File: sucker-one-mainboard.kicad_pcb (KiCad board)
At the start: 4 copper layers, 79.4 x 63 mm, 114 parts, among them J1 JST NC Valve, J10 JST Motor, J11 User Interface Module, J12 SWD, J2 JST NO Valve, J3 6P4C, J4 JST 3 Way Valve, J5 AUX SPI, J6 AUX I2C, Q1 BSS138, Q2 BSS138, Q3 BSS138, Q4 DMN15H310SE-13, SW1 Power Switch, SW2 Reset, U1 LD1117S33TR, U2 TPS61087DRCR, U3 STM32F103RBTx, U4 2SMPP-03, U5 INA125UA, Y1 8MHz(16pf)

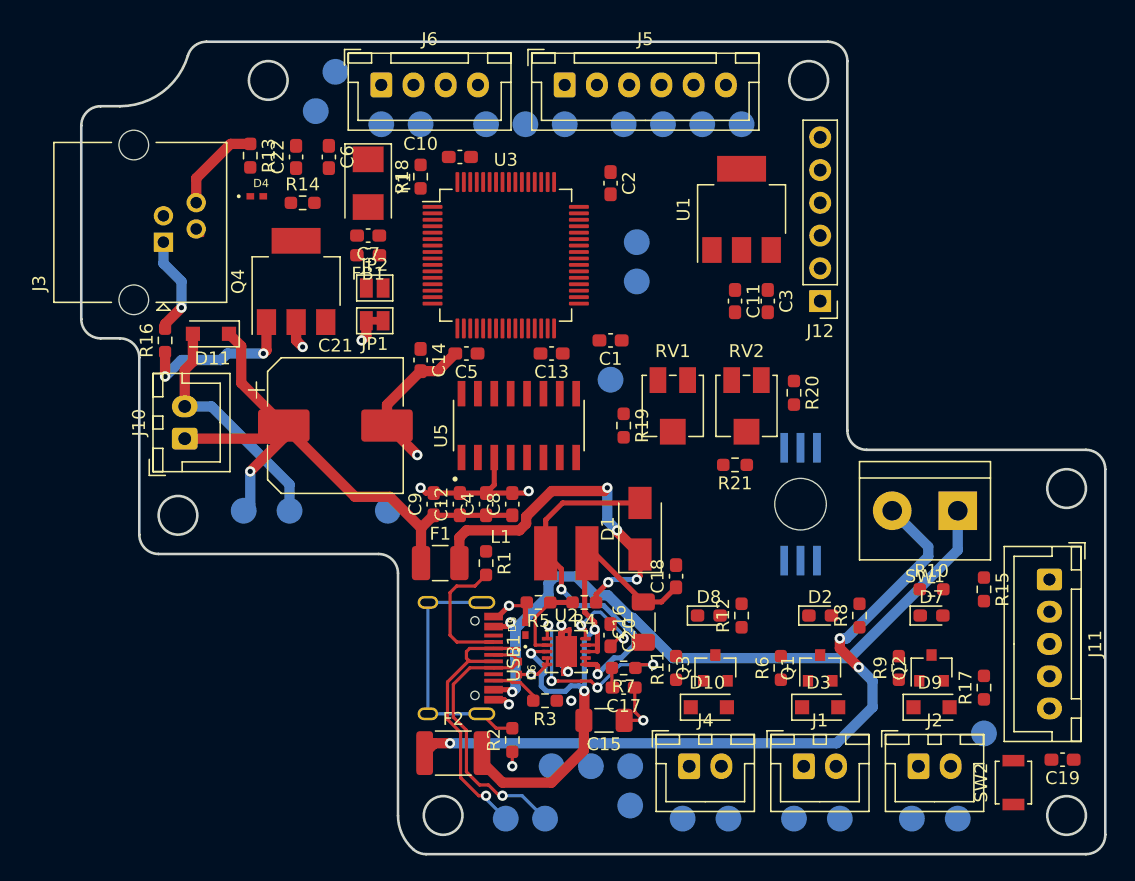
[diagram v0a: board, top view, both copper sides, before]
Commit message: routing finished
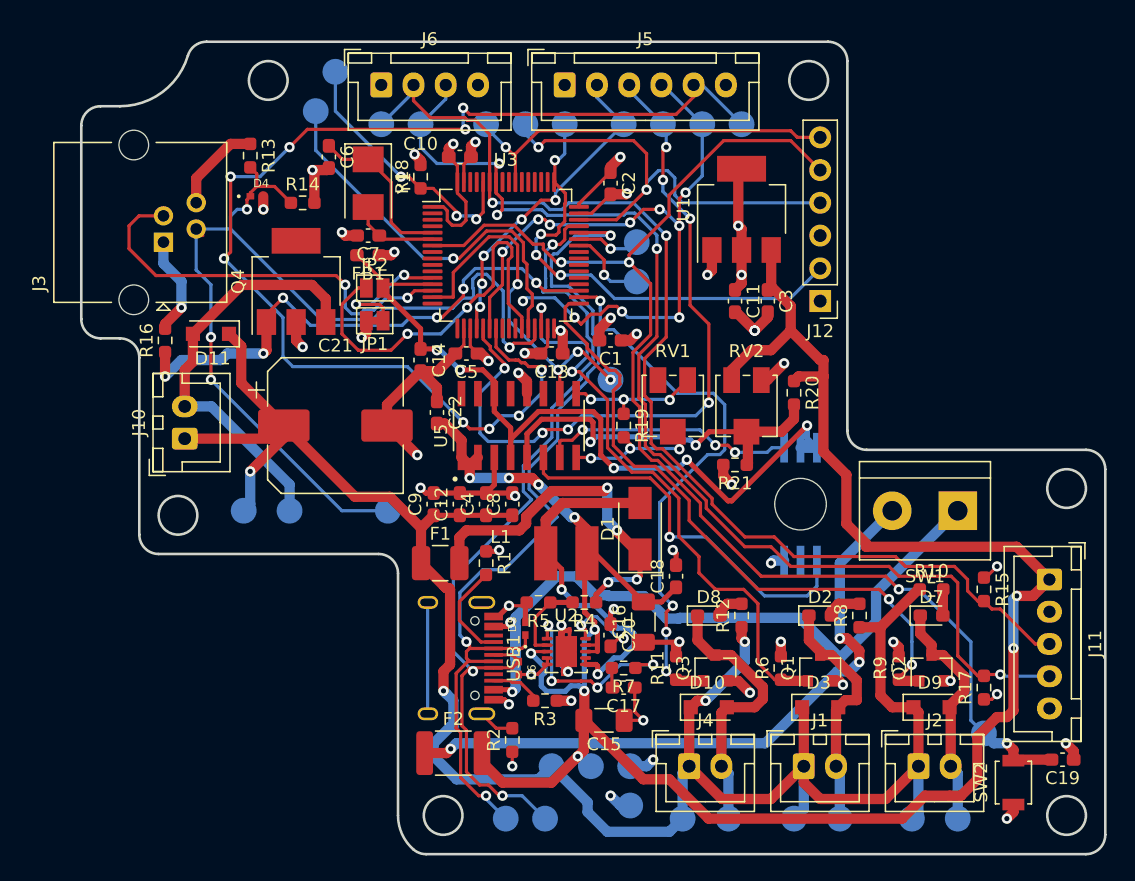
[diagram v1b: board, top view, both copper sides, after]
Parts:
- moved C22 22.6 mm to (84.6, 79.2), turned to 270 degrees
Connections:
- U2 pad 11: GNDA -> GND
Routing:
- net VBUS: track 47.2 -> 172.5 mm, vias 3 -> 10
- net +12V: track 49.0 -> 162.3 mm, vias 1 -> 4
- net NRST: track 0.00 -> 100.7 mm, vias 0 -> 4
- net SPI1_MOSI: track 0.00 -> 93.6 mm, vias 0 -> 9
- net I2C1_SCL: track 0.00 -> 89.8 mm, vias 0 -> 4
- net I2C1_SDA: track 0.00 -> 87.8 mm, vias 0 -> 2
- net FOOTPEDAL: track 0.72 -> 77.5 mm, vias 0 -> 4
- net VDDA: track 0.00 -> 64.6 mm, vias 0 -> 5
- net GND: track 50.7 -> 114.2 mm, vias 12 -> 41
- net SPI1_MISO: track 0.00 -> 56.4 mm, vias 0 -> 11
- net SPI1_CLK: track 0.00 -> 56.3 mm, vias 0 -> 7
- net NO_VALVE: track 0.00 -> 50.4 mm, vias 0 -> 2
- net D-: track 22.1 -> 71.0 mm, vias 1 -> 3
- net NC_VALVE: track 0.00 -> 45.8 mm, vias 0 -> 2
- net D+: track 22.8 -> 67.4 mm, vias 1 -> 3
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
